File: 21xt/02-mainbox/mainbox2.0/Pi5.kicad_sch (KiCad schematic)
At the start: 4 parts, among them J12 Conn_02x20_Odd_Even

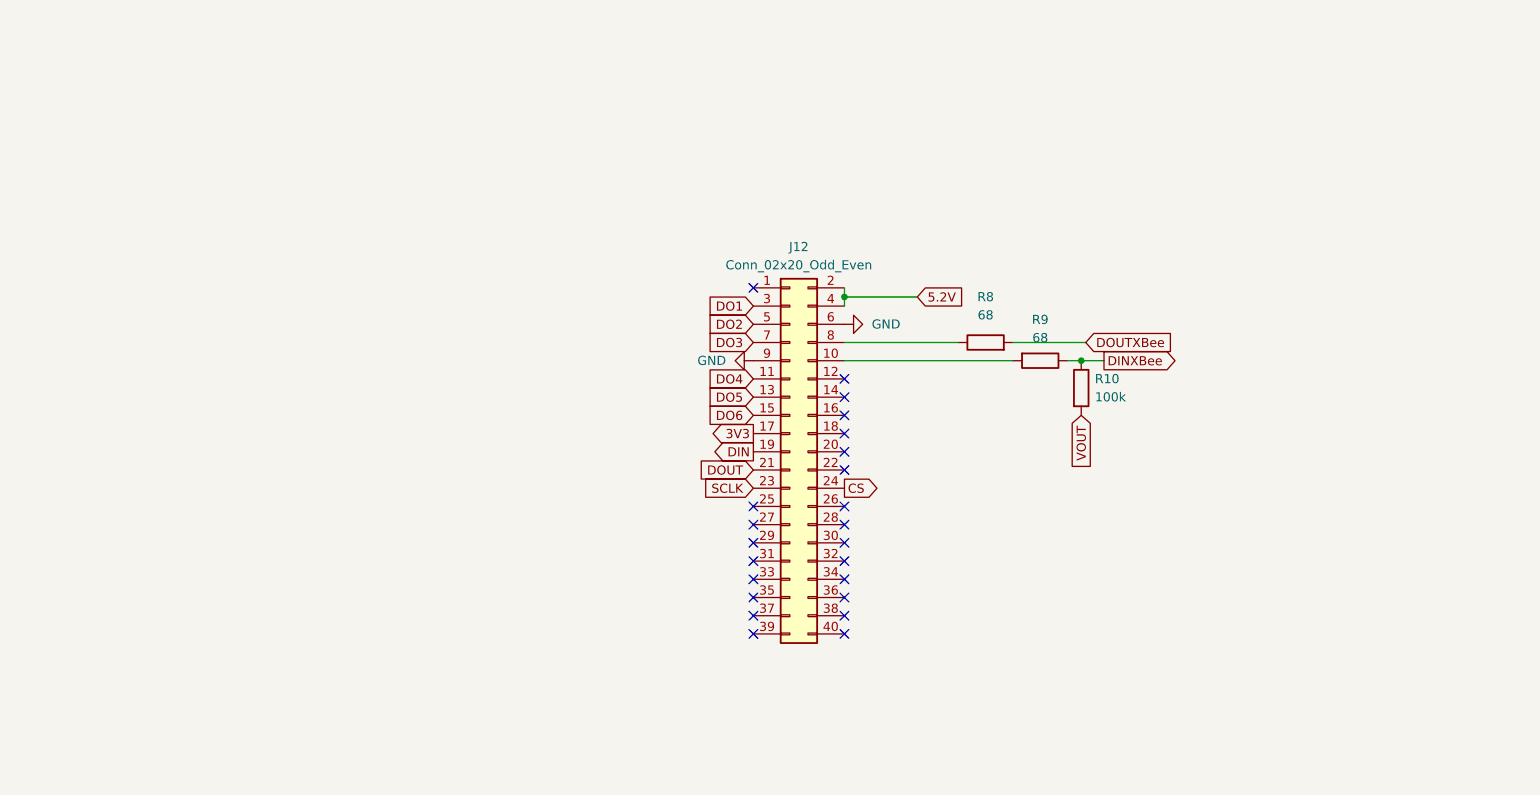
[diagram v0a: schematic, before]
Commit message: schematic check
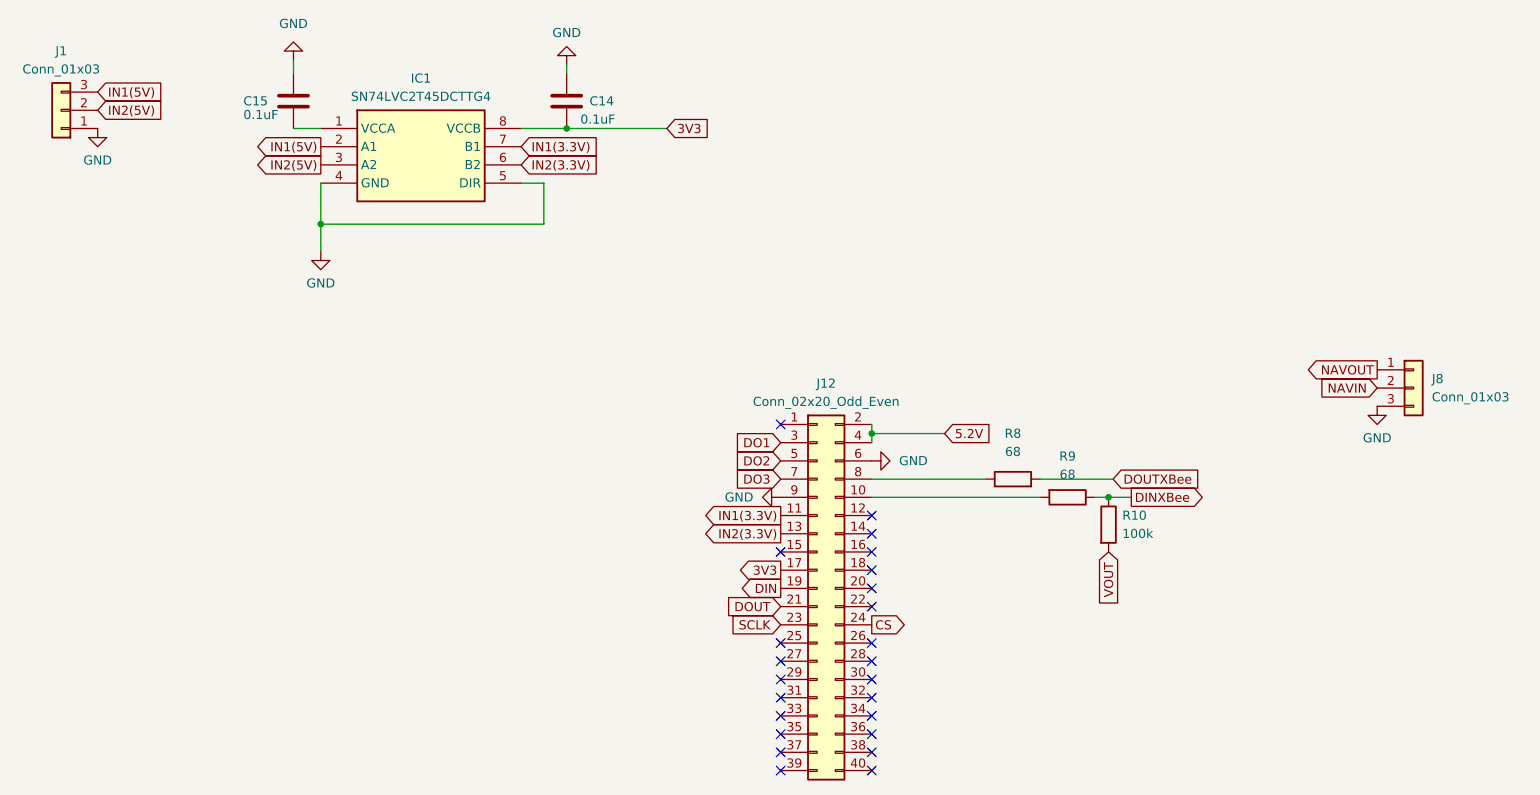
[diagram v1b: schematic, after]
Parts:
- added C14, C15: 0.1uF, symbol Device:C
- added IC1: SN74LVC2T45DCTTG4, symbol Logic_LevelTranslator:SN74LVC2T45DCTTG4
- added J1, J8: Conn_01x03, symbol Connector_Generic:Conn_01x03
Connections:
- net 3V3: now also C14.2, IC1.8 (VCCB)
- net GND: now also C14.1, C15.1, IC1.4 (GND), IC1.5 (DIR), J1.1 (Pin_1), J8.3 (Pin_3)
- net DO4 renamed IN1(3.3V)
- net IN1(3.3V): now also IC1.7 (B1)
- net DO5 renamed IN2(3.3V)
- net IN2(3.3V): now also IC1.6 (B2)
- net DO6: no longer names the net of J12.15 (Pin_15)
- new net: C15.2, IC1.1 (VCCA)
- new net IN1(5V): IC1.2 (A1), J1.3 (Pin_3)
- new net IN2(5V): IC1.3 (A2), J1.2 (Pin_2)
- new net NAVIN: J8.2 (Pin_2)
- new net NAVOUT: J8.1 (Pin_1)
- no-connect marks 23 -> 24
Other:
- moved on the sheet: J12, R10, R8, R9
